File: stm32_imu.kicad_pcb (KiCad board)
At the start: 4 copper layers, 26 x 42.5 mm, 44 parts, among them J1 USB_C_Receptacle_USB2.0_16P, J3 TC2030, U1 NRF24L01, U3 LM1117MP-3.3, U4 2.4GHz, U5 ICM-20948, U6 STM32F411CEUx, Y1 16MHz, Y2 24MHz

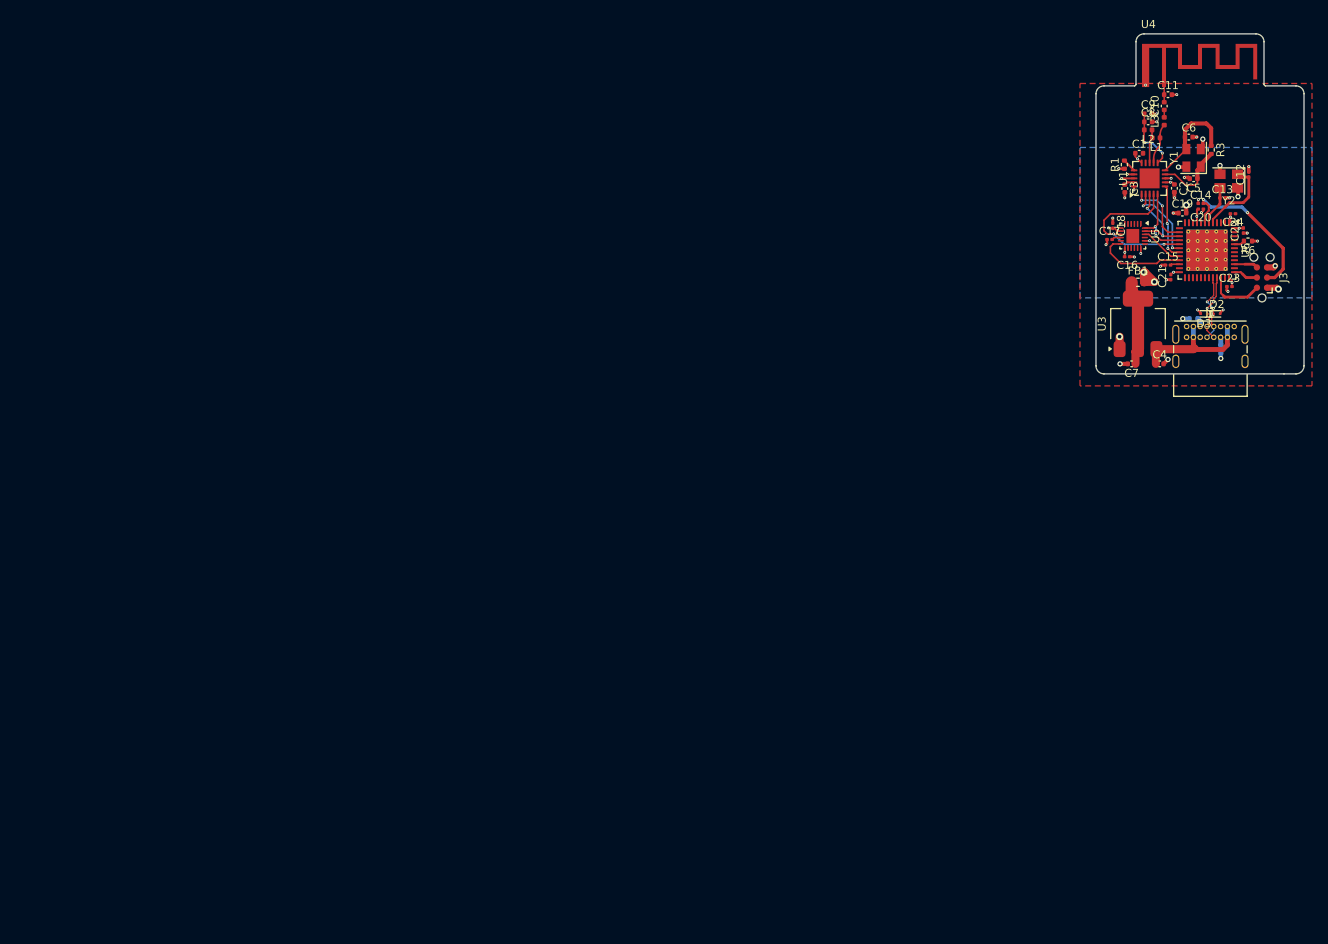
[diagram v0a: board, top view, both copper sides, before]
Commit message: Add files via upload
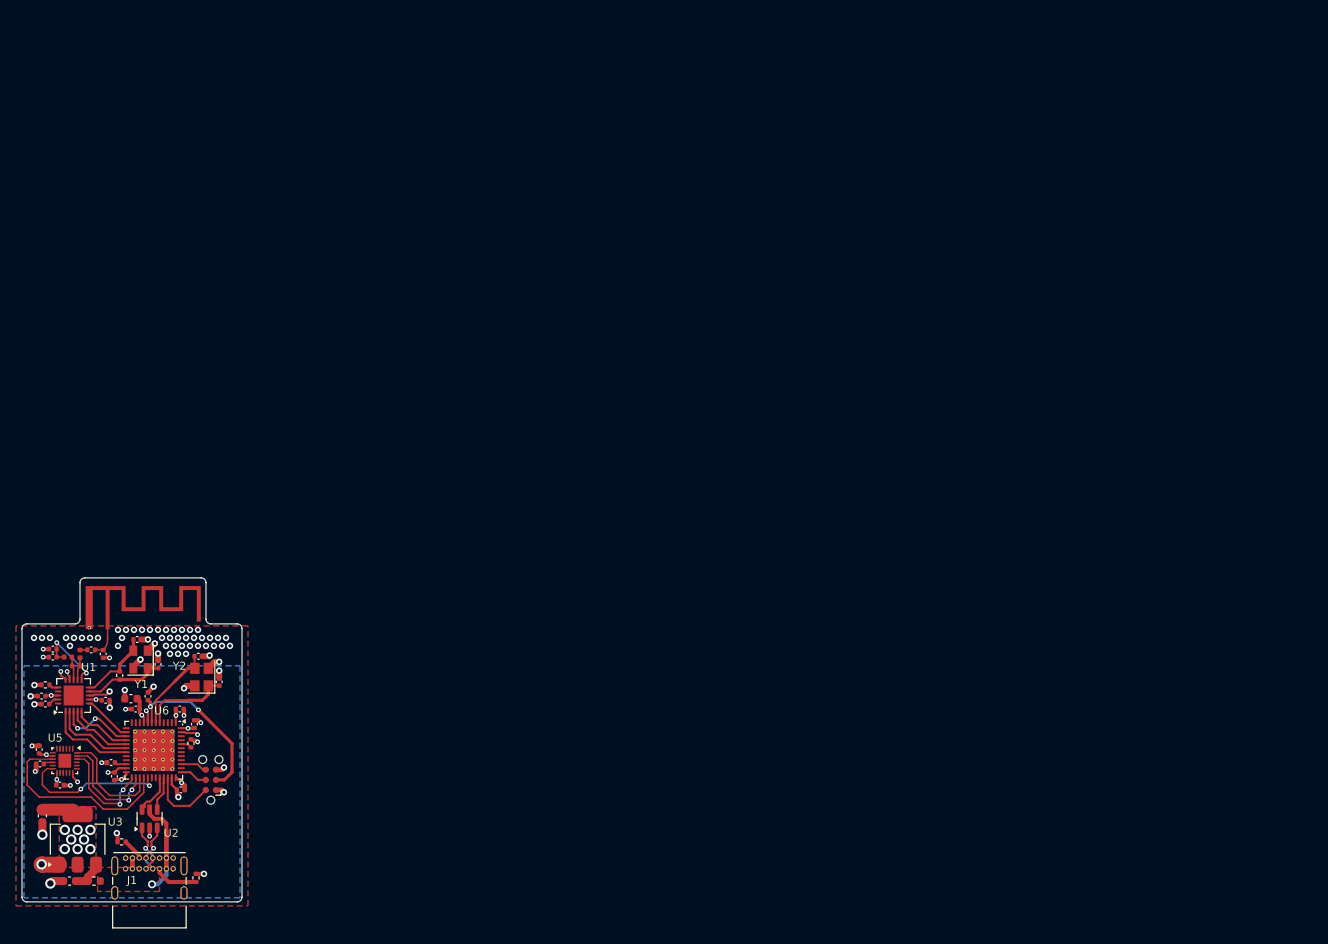
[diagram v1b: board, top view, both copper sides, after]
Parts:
- removed D2, D3: ESD, Diode_SMD:D_SOD-923
- added U2: USBLC6-2SC6, Package_TO_SOT_SMD:SOT-23-6, F.Cu at (100.7, 174.1)
- C12, C13, C14, C15, C16, C17, C18, C20, C21, C22, C23, C24: footprint Capacitor_SMD:C_0201_0603Metric -> Capacitor_SMD:C_0402_1005Metric
- C19: footprint Capacitor_SMD:C_0402_1005Metric -> Capacitor_SMD:C_0603_1608Metric
- C4, C7: value 22u -> 10u; footprint Capacitor_SMD:C_0402_1005Metric -> Capacitor_SMD:C_0603_1608Metric
- FB1: value 600 @ 100MHz -> 100 @ 100MHz
- R4, R5: moved to F.Cu
- moved C1 153.1 mm to (87.2, 158.8), turned to 180 degrees
- moved C9 152.8 mm to (88.6, 153.9), turned to 180 degrees
- moved C23 152.2 mm to (96.3, 168.8), turned to -90 degrees
- moved C8 152.0 mm to (88.6, 152.9), turned to 180 degrees
- moved R3 151.4 mm to (97.0, 156.2)
- moved L3 151.0 mm to (92.0, 153.5)
- moved C4 150.8 mm to (90.7, 181.9), turned to 180 degrees
- moved FB1 150.4 mm to (93.8, 181.9), turned to 180 degrees
- moved C10 150.4 mm to (93.4, 153.0), turned to 0 degrees
- moved C11 150.3 mm to (94.9, 153.5), turned to -90 degrees
- moved L1 150.3 mm to (91.5, 155.0)
- moved L2 150.2 mm to (90.5, 153.9)
- moved R1 149.7 mm to (87.7, 157.4), turned to 0 degrees
- moved C3 149.5 mm to (87.7, 159.8), turned to 180 degrees
- moved C18 149.3 mm to (86.9, 165.5)
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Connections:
- net SPI1_CS0 renamed SPI1_CS
- C4 pad 1: VBUS -> Net-(U3-VI)
- C7 pad 1: /VREG_O -> +3.3V
- FB1 pad 1: /VREG_O -> VBUS
- FB1 pad 2: +3.3V -> Net-(U3-VI)
- J1 pad A6: D+ -> CONN_D+
- J1 pad A7: D- -> CONN_D-
- J1 pad B6: D+ -> CONN_D+
- J1 pad B7: D- -> CONN_D-
- J1 pad S1: GND -> unconnected-(J1-SHIELD-PadS1)_2
- U3 pad 2: /VREG_O -> +3.3V
- U3 pad 3: VBUS -> Net-(U3-VI)
- U5 pad 12: INT1 -> IMU_INT
- U5 pad 22: SPI1_CS1 -> SPI2_CS
- U5 pad 23: SPI1_SCK -> SPI2_SCK
- U5 pad 24: SPI1_MISO -> SPI2_MISO
- U5 pad 9: SPI1_MOSI -> SPI2_MOSI
- U6 pad 14: CE -> IRQ
- U6 pad 19: IRQ -> CE
- U6 pad 20: SPI1_CS1 -> unconnected-(U6-PB2-Pad20)
- U6 pad 21: INT1 -> unconnected-(U6-PB10-Pad21)
- U6 pad 25: unconnected-(U6-PB12-Pad25) -> SPI2_CS
- U6 pad 26: unconnected-(U6-PB13-Pad26) -> SPI2_SCK
- U6 pad 27: unconnected-(U6-PB14-Pad27) -> SPI2_MISO
- U6 pad 28: unconnected-(U6-PB15-Pad28) -> SPI2_MOSI
- U6 pad 29: unconnected-(U6-PA8-Pad29) -> IMU_INT
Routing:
- net SPI2_MOSI: track 0.00 -> 24.8 mm
- net GND: track 28.4 -> 48.6 mm, vias 39 -> 83
- net IMU_INT: track 0.00 -> 18.5 mm, vias 0 -> 2
- net SPI2_SCK: track 0.00 -> 13.8 mm, vias 0 -> 2
- net SPI2_MISO: track 0.00 -> 13.7 mm
- net SPI2_CS: track 0.00 -> 13.5 mm, vias 0 -> 2
- net SPI1_MOSI: track 21.0 -> 8.48 mm, vias 2 -> 0
- net INT1: track 11.6 -> 0.00 mm
- net /VREG_O: track 10.7 -> 0.00 mm
- net CONN_D+: track 0.00 -> 6.29 mm, vias 0 -> 1
- net CONN_D-: track 0.00 -> 6.27 mm, vias 0 -> 1
- net RCC_OSC_OUT: track 4.93 -> 10.8 mm
- net SPI1_CS1: track 5.46 -> 0.00 mm
- net CC2: track 0.98 -> 5.52 mm
- net D+: track 8.51 -> 4.32 mm, vias 2 -> 0
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- added copper zone on F.Cu, net +3.3V
- added copper zone on F.Cu, net VBUS
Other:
- board size 26 x 42.5 mm -> 27.5 x 40.5 mm
